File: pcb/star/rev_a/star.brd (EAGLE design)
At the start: 46.2 x 40 mm, 42 parts, among them J2 TC2030-JLINK-NL, J3 MICRO_USB_B_HIROSE_ZX62-B-5PA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, J4 TC2030-JLINK-NL, U2 LTC4065, U3 TRIPOINT, U4 TPS715AXX, U5 NRF51822QF, X1 EPSON-FA-128

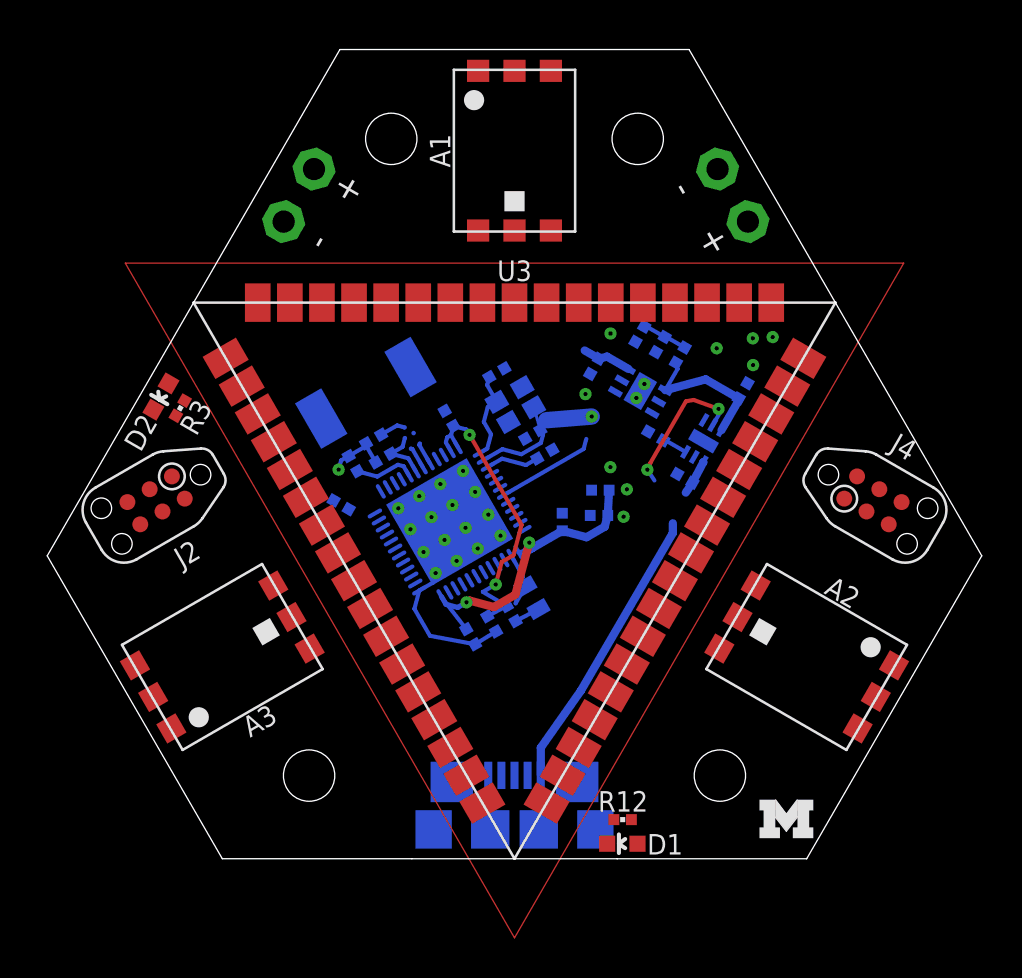
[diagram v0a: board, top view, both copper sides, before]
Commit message: tag coming along
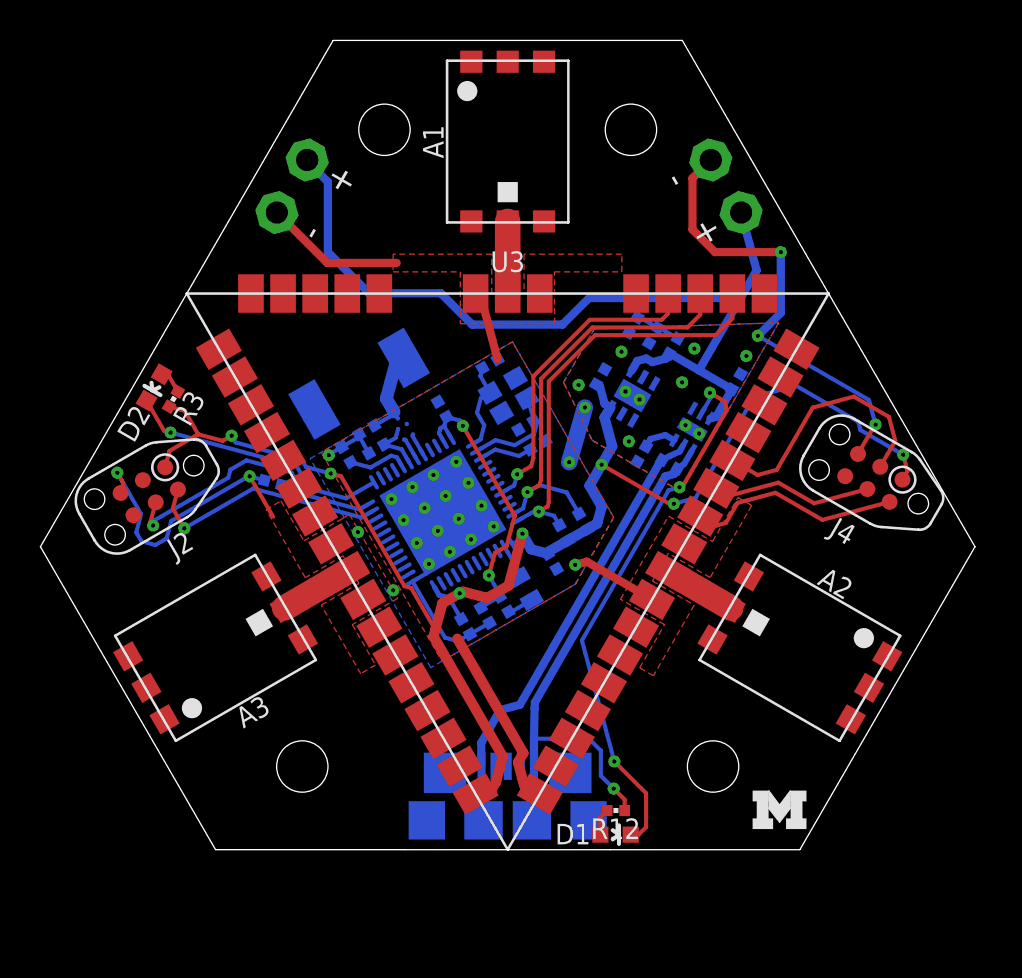
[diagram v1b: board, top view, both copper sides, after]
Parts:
- D1: value (none) -> GREEN
- D2: value (none) -> BLUE
- moved R6 3.55 mm to (-12.0, 0.27), turned to 195 degrees
- moved C14 2.01 mm to (1.87, -3.63), turned to 240 degrees
- moved R1 1.94 mm to (2.44, -2.21), turned to 240 degrees
- moved R2 1.76 mm to (3.41, -1.65), turned to 240 degrees
- moved R10 1.13 mm to (6.29, 1.68), turned to 120 degrees
- moved J4 1.11 mm to (17.8, 0.50), turned to 150 degrees
- moved C18 1.02 mm to (7.68, 1.17)
- moved U2 0.80 mm to (8.80, 2.90)
- moved C17 0.60 mm to (4.26, 5.50), turned to 120 degrees
- moved L1 0.59 mm to (-0.51, -5.74)
- moved L3 0.56 mm to (0.53, -4.98)
- moved LOGO1 0.56 mm to (11.8, -16.9)
- moved D1 0.56 mm to (5.00, -17.1), turned to 270 degrees
- moved R12 0.56 mm to (5.02, -16.0), turned to 0 degrees
- moved A2 0.56 mm to (14.1, -7.91)
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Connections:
- new net N$1: A3.A, U3.9
- new net N$2: A2.A, U3.26
- new net N$3: A1.A, U3.43
- new net N$4: J4.2, U3.28
- new net N$7: J4.4, U3.29
- new net N$8: J4.3, U3.30
- net DW_INT: now also U3.38
- net GND: now also U3.10, U3.18, U3.25, U3.27, U3.42, U3.44, U3.8
- net I2C_SCL: now also U3.37
- net I2C_SDA: now also U3.36
- net N$6: now also U5.25; no longer U5.43
- net VCC: now also U3.17
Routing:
- net VCC: track 18.3 -> 76.2 mm, vias 2 -> 7
- net VBAT: track 7.30 -> 43.9 mm
- net GND: track 128.1 -> 93.3 mm, vias 27 -> 35
- net I2C_SCL: track 0.00 -> 20.9 mm, vias 0 -> 1
- net I2C_SDA: track 0.00 -> 20.8 mm, vias 0 -> 1
- net N$5: track 7.15 -> 27.1 mm, vias 2 -> 3
- net DW_INT: track 0.00 -> 15.5 mm, vias 0 -> 1
- net SWDCLK: track 0.00 -> 14.7 mm, vias 0 -> 1
- net N$8: track 0.00 -> 12.8 mm
- net SWDIO/!RESET: track 0.00 -> 12.2 mm, vias 0 -> 1
- net N$4: track 0.00 -> 10.6 mm
- net VUSB: track 16.1 -> 25.0 mm, vias 0 -> 1
- net N$6: track 5.06 -> 13.3 mm, vias 0 -> 1
- net N$7: track 0.00 -> 8.03 mm
- net N$1: track 0.00 -> 3.58 mm
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- added copper zone on layer 1, net GND
- added copper zone on layer 16, net GND
